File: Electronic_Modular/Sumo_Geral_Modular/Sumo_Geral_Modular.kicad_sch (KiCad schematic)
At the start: 50 parts, among them J1 Bateria, J10 ESC1, J11 ESC2, J12 USB_B_Micro, J13 ADSN-9500, J14 PS ADSN-9500, J15 MPU-6050, J2 VL53L0X 1, J3 VL53L0X 2, J4 VL53L0X 3, J5 VS1838B, J8 Motor A, J9 Motor B, Q1 S8050, Q2 S8050, SW2 EN, SW3 BOOT, U1 AMS1117-5.0, U2 AMS1117-3.3, U3 CH340C

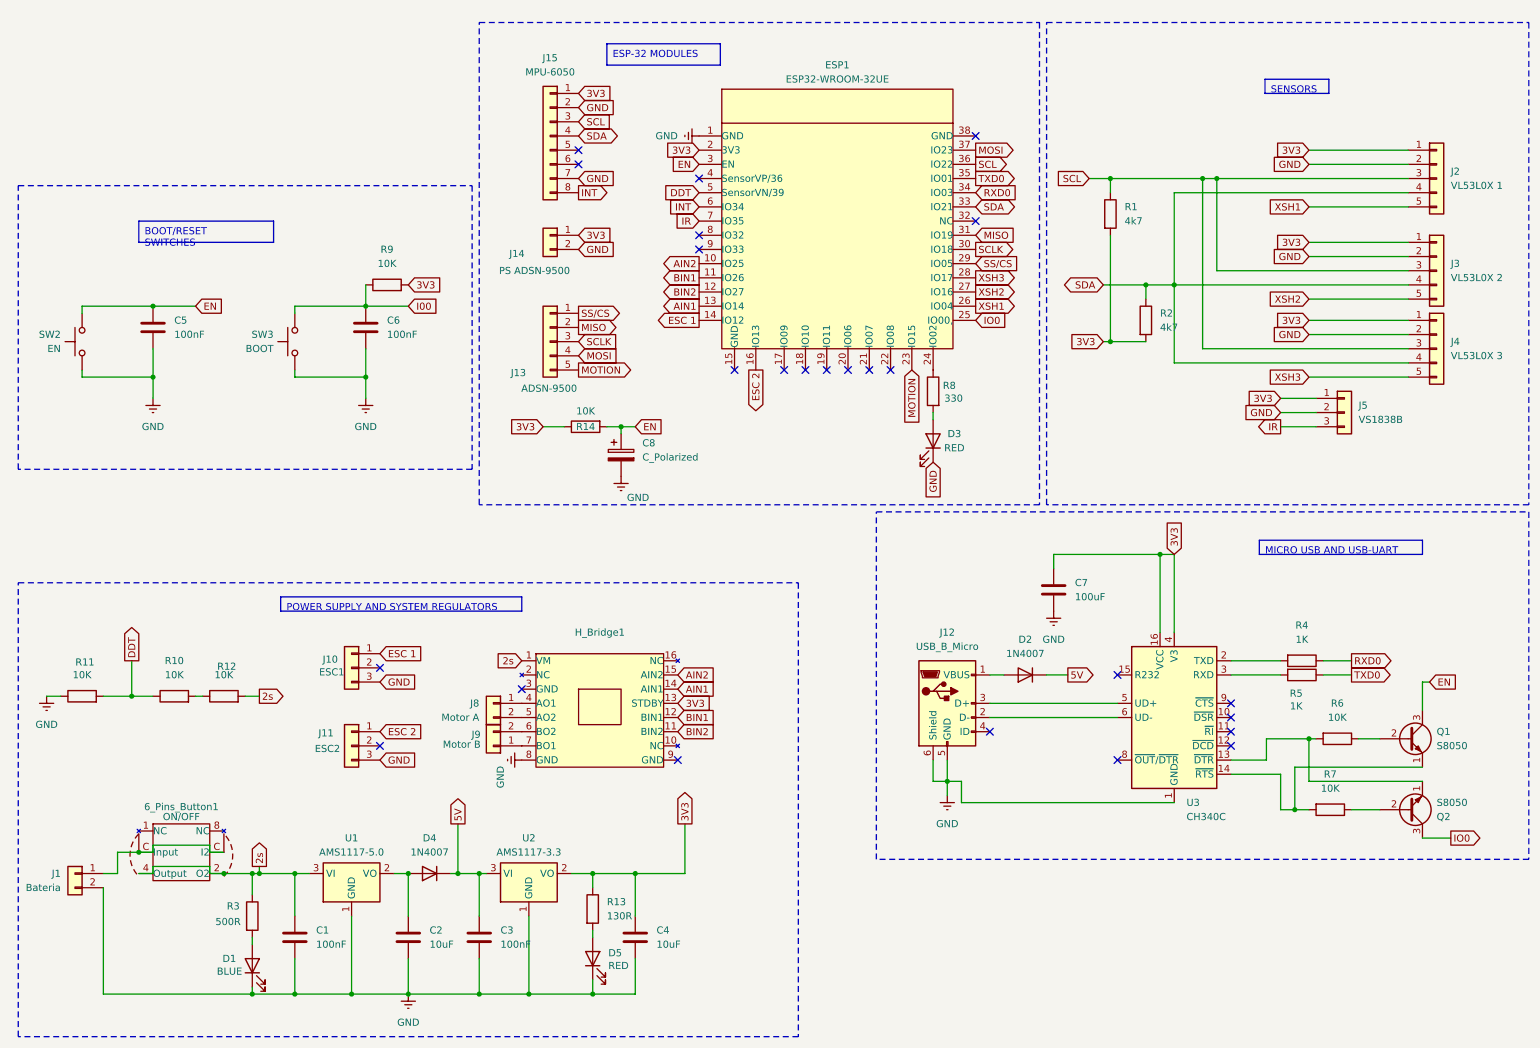
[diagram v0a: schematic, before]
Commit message: chore: schamatic review
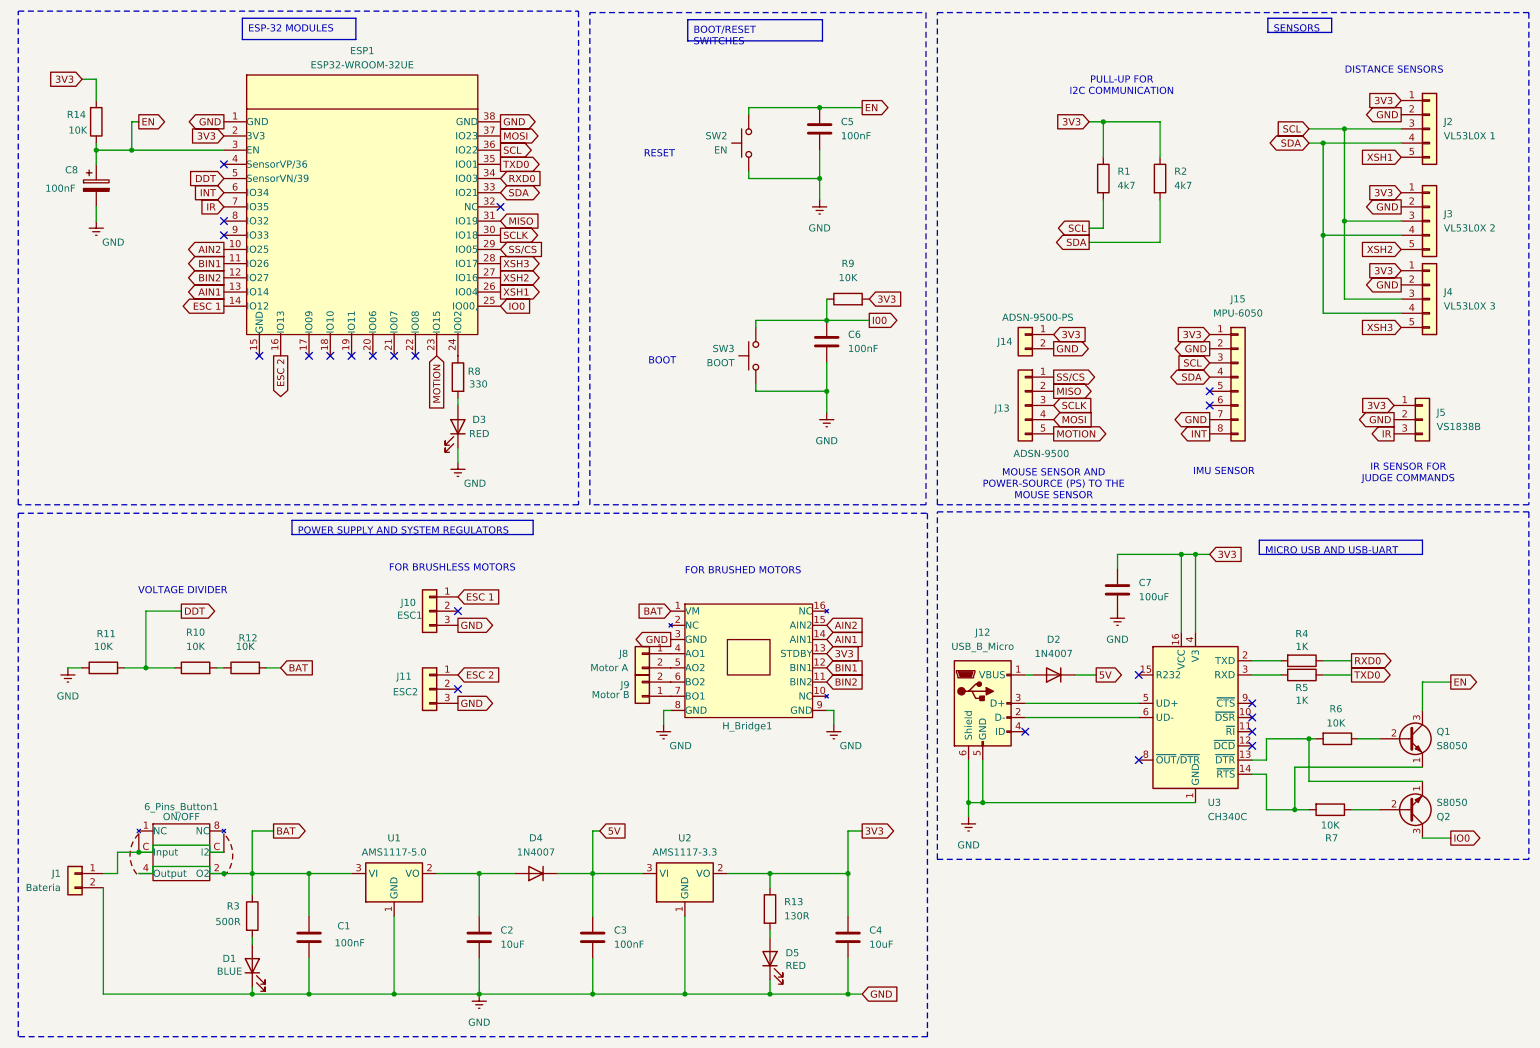
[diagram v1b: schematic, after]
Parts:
- C8: value C_Polarized -> 100nF
- J14: value PS ADSN-9500 -> ADSN-9500-PS
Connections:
- net 3V3: now also R1.1, R14.2, R2.1; no longer R1.2, R14.1, R2.2
- net EN: now also R14.1; no longer R14.2
- net GND: now also ESP1.38 (GND), H_Bridge1.3 (GND), H_Bridge1.9 (GND)
- net SCL: now also R1.2; no longer R1.1
- net SDA: now also R2.2; no longer R2.1
- net 2s renamed BAT
- no-connect marks 25 -> 22
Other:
- note added: "BOOT"
- note added: "DISTANCE SENSORS"
- note added: "FOR BRUSHED MOTORS"
- note added: "FOR BRUSHLESS MOTORS"
- note added: "IMU SENSOR"
- note added: "IR SENSOR FOR JUDGE COMMANDS"
- note added: "MOUSE SENSOR AND POWER-SOURCE (PS) TO THE MOUSE SENSOR"
- note added: "PULL-UP FOR I2C COMMUNICATION"
- note added: "RESET"
- note added: "VOLTAGE DIVIDER"
- company: (none) -> PROJECT NEON
- title: (none) -> MODULAR PCB FOR MINI SUMO ROBOTS
- moved on the sheet: C1, C2, C3, C4, C5, C6, C7, C8, D2, D3, D4, D5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

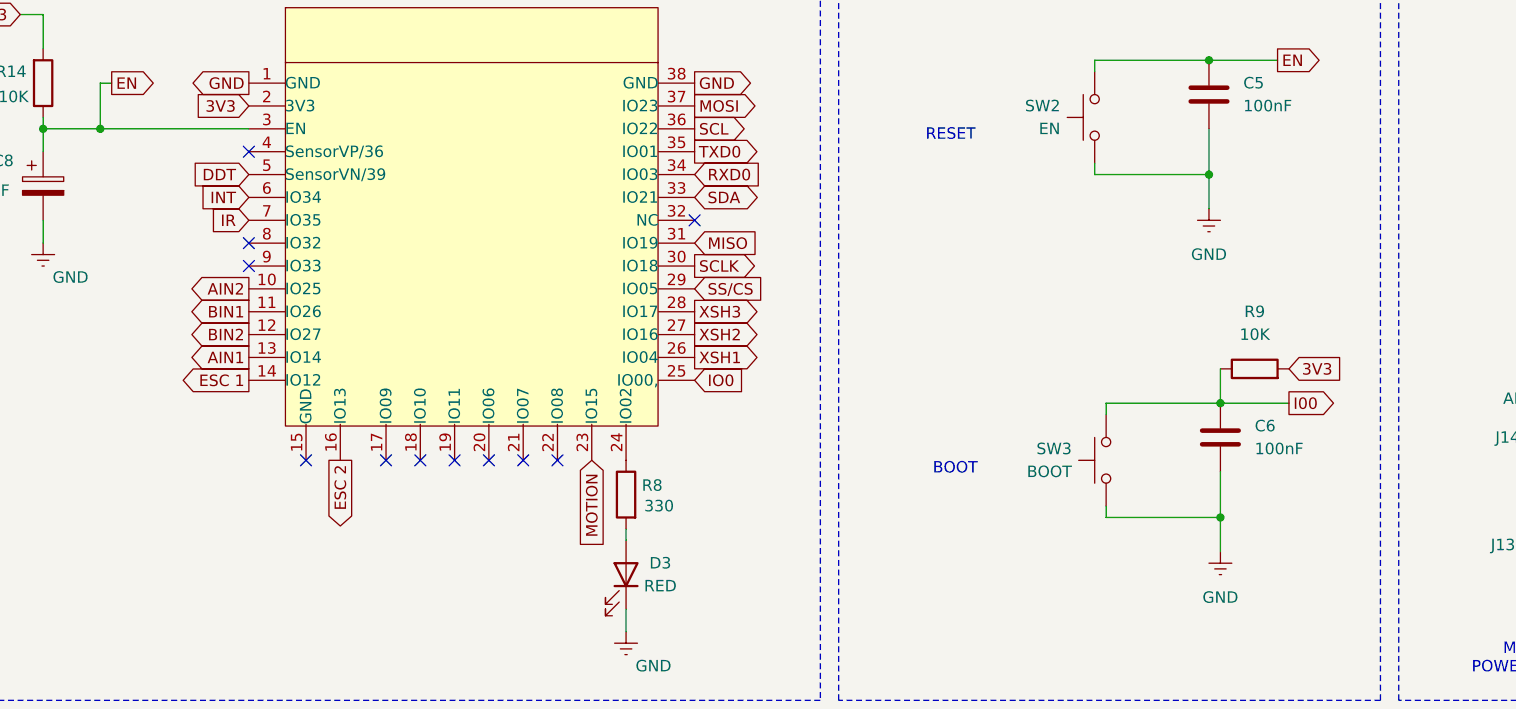
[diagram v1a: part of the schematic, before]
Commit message: chore: finish PCB V1
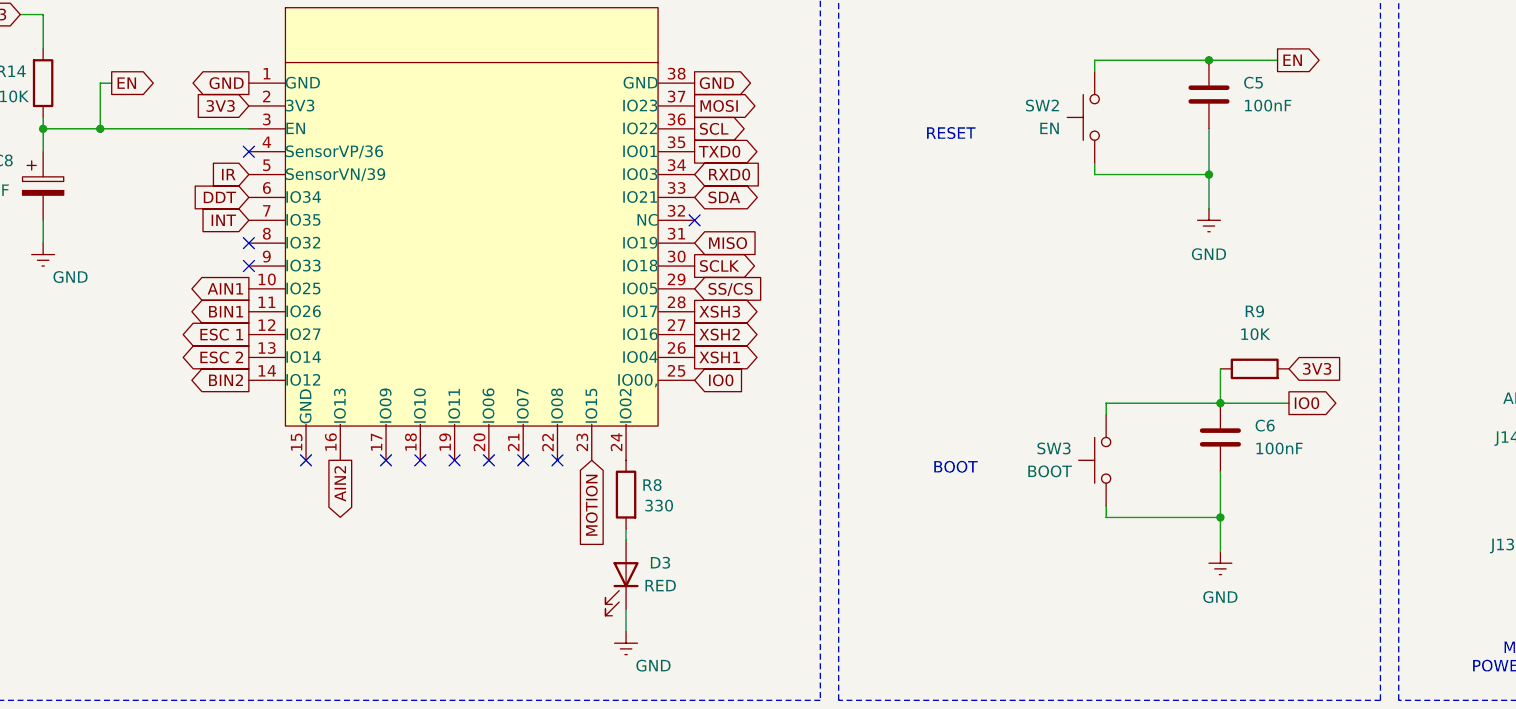
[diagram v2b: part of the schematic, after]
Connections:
- net I00 is gone; now on net IO0: C6.1, R9.1, SW3.1
- net AIN1: now also ESP1.10 (IO25); no longer ESP1.13 (IO14)
- net AIN2: now also ESP1.16 (IO13); no longer ESP1.10 (IO25)
- net BIN2: now also ESP1.14 (IO12); no longer ESP1.12 (IO27)
- net DDT: now also ESP1.6 (IO34); no longer ESP1.5 (SensorVN/39)
- net ESC 1: now also ESP1.12 (IO27); no longer ESP1.14 (IO12)
- net ESC 2: now also ESP1.13 (IO14); no longer ESP1.16 (IO13)
- net INT: now also ESP1.7 (IO35); no longer ESP1.6 (IO34)
- net IR: now also ESP1.5 (SensorVN/39); no longer ESP1.7 (IO35)
